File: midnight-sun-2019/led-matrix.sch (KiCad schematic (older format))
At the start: 826 parts

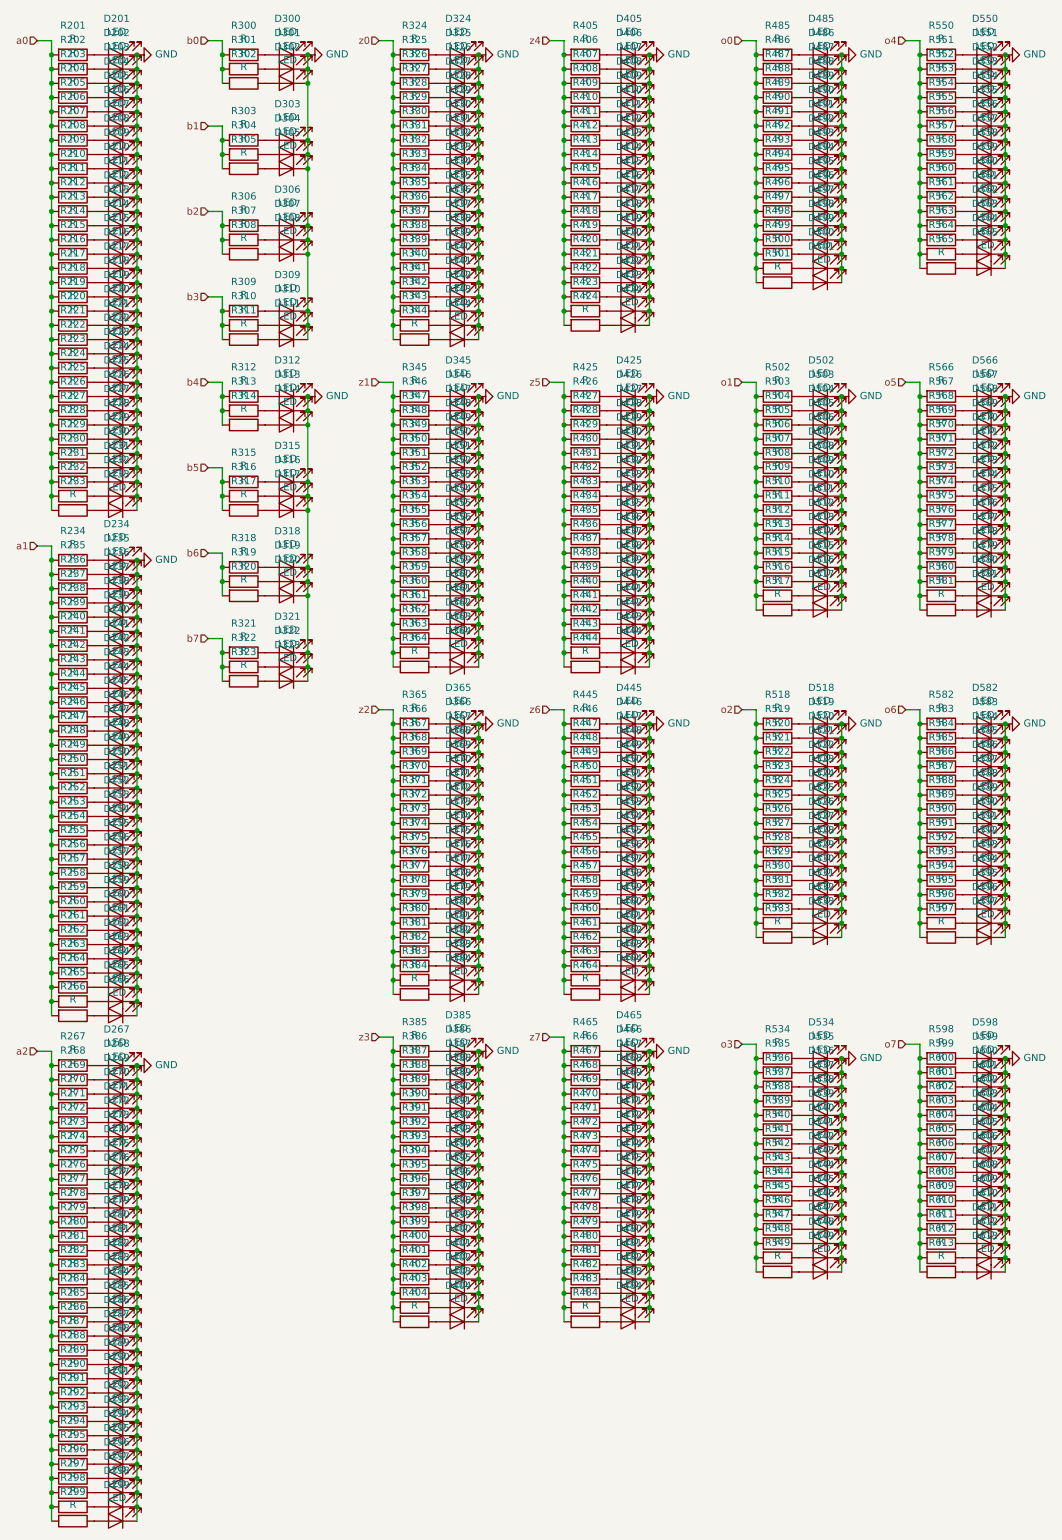
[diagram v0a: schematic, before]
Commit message: Clean up circuit draft
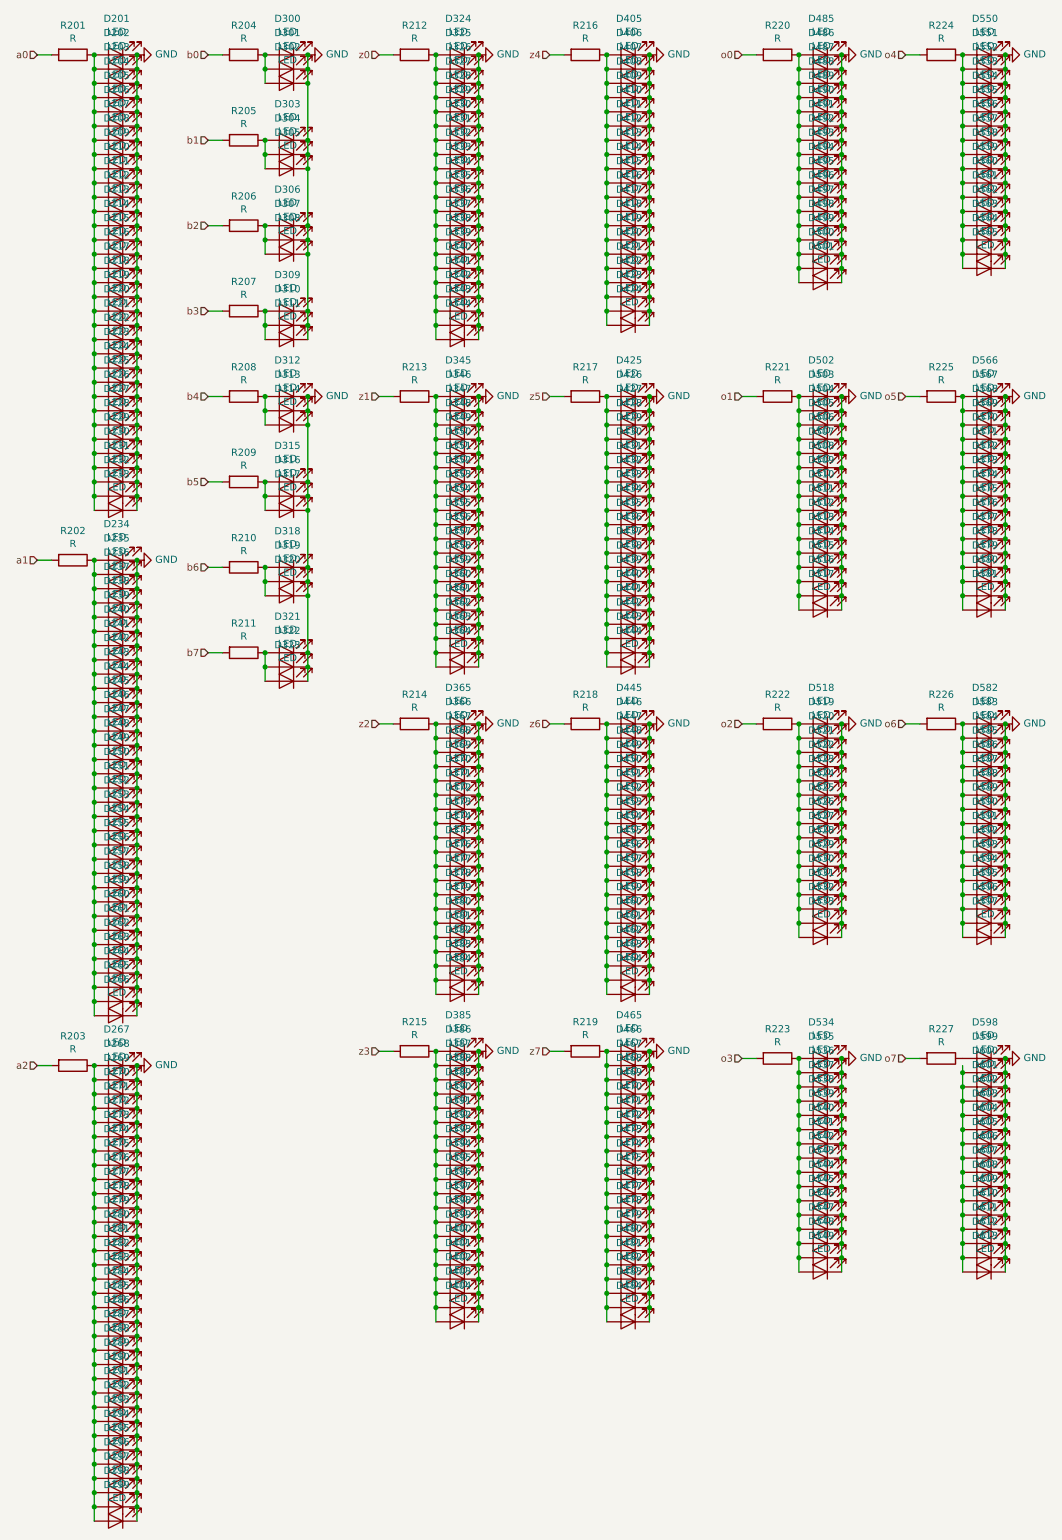
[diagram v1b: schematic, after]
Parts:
- removed R202, R203, R204, R205, R206, R207, R208, R209, R210, R211, R212, R213, R214, R215, R216, R217, R218, R219, R220, R221, R222, R223, R224, R225, R226, R227, R228, R229, R230, R231, R232, R233, R235, R236, R237, R238, R239, R240, R241, R242, R243, R244, R245, R246, R247, R248, R249, R250, R251, R252, R253, R254, R255, R256, R257, R258, R259, R260, R261, R262, R263, R264, R265, R266, R268, R269, R270, R271, R272, R273, R274, R275, R276, R277, R278, R279, R280, R281, R282, R283, R284, R285, R286, R287, R288, R289, R290, R291, R292, R293, R294, R295, R296, R297, R298, R299, R301, R302, R304, R305, R307, R308, R310, R311, R313, R314, R316, R317, R319, R320, R322, R323, R325, R326, R327, R328, R329, R330, R331, R332, R333, R334, R335, R336, R337, R338, R339, R340, R341, R342, R343, R344, R346, R347, R348, R349, R350, R351, R352, R353, R354, R355, R356, R357, R358, R359, R360, R361, R362, R363, R364, R366, R367, R368, R369, R370, R371, R372, R373, R374, R375, R376, R377, R378, R379, R380, R381, R382, R383, R384, R386, R387, R388, R389, R390, R391, R392, R393, R394, R395, R396, R397, R398, R399, R400, R401, R402, R403, R404, R406, R407, R408, R409, R410, R411, R412, R413, R414, R415, R416, R417, R418, R419, R420, R421, R422, R423, R424, R426, R427, R428, R429, R430, R431, R432, R433, R434, R435, R436, R437, R438, R439, R440, R441, R442, R443, R444, R446, R447, R448, R449, R450, R451, R452, R453, R454, R455, R456, R457, R458, R459, R460, R461, R462, R463, R464, R466, R467, R468, R469, R470, R471, R472, R473, R474, R475, R476, R477, R478, R479, R480, R481, R482, R483, R484, R486, R487, R488, R489, R490, R491, R492, R493, R494, R495, R496, R497, R498, R499, R500, R501, R503, R504, R505, R506, R507, R508, R509, R510, R511, R512, R513, R514, R515, R516, R517, R519, R520, R521, R522, R523, R524, R525, R526, R527, R528, R529, R530, R531, R532, R533, R535, R536, R537, R538, R539, R540, R541, R542, R543, R544, R545, R546, R547, R548, R549, R551, R552, R553, R554, R555, R556, R557, R558, R559, R560, R561, R562, R563, R564, R565, R567, R568, R569, R570, R571, R572, R573, R574, R575, R576, R577, R578, R579, R580, R581, R583, R584, R585, R586, R587, R588, R589, R590, R591, R592, R593, R594, R595, R596, R597, R599, R600, R601, R602, R603, R604, R605, R606, R607, R608, R609, R610, R611, R612, R613: R, symbol Device:R
- renumbered R234 to R202, R267 to R203, R300 to R204, R303 to R205, R306 to R206, R309 to R207, R312 to R208, R315 to R209, R318 to R210, R321 to R211, R324 to R212, R345 to R213, R365 to R214, R385 to R215, R405 to R216, R425 to R217, R445 to R218, R465 to R219, R485 to R220, R502 to R221, R518 to R222, R534 to R223, R550 to R224, R566 to R225, R582 to R226, R598 to R227
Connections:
- net at D612.2 (A): now also D599.2 (A), D600.2 (A), D601.2 (A), D602.2 (A), D603.2 (A), D604.2 (A), D605.2 (A), D606.2 (A), D607.2 (A), D608.2 (A), D609.2 (A), D610.2 (A), D611.2 (A), D613.2 (A)
- net at D596.2 (A): now also D582.2 (A), D583.2 (A), D584.2 (A), D585.2 (A), D586.2 (A), D587.2 (A), D588.2 (A), D589.2 (A), D590.2 (A), D591.2 (A), D592.2 (A), D593.2 (A), D594.2 (A), D595.2 (A), D597.2 (A), R226.1
- net at D580.2 (A): now also D566.2 (A), D567.2 (A), D568.2 (A), D569.2 (A), D570.2 (A), D571.2 (A), D572.2 (A), D573.2 (A), D574.2 (A), D575.2 (A), D576.2 (A), D577.2 (A), D578.2 (A), D579.2 (A), D581.2 (A), R225.1
- net at D564.2 (A): now also D550.2 (A), D551.2 (A), D552.2 (A), D553.2 (A), D554.2 (A), D555.2 (A), D556.2 (A), D557.2 (A), D558.2 (A), D559.2 (A), D560.2 (A), D561.2 (A), D562.2 (A), D563.2 (A), D565.2 (A), R224.1
- net at D548.2 (A): now also D534.2 (A), D535.2 (A), D536.2 (A), D537.2 (A), D538.2 (A), D539.2 (A), D540.2 (A), D541.2 (A), D542.2 (A), D543.2 (A), D544.2 (A), D545.2 (A), D546.2 (A), D547.2 (A), D549.2 (A), R223.1
- net at D532.2 (A): now also D518.2 (A), D519.2 (A), D520.2 (A), D521.2 (A), D522.2 (A), D523.2 (A), D524.2 (A), D525.2 (A), D526.2 (A), D527.2 (A), D528.2 (A), D529.2 (A), D530.2 (A), D531.2 (A), D533.2 (A), R222.1
- net at D516.2 (A): now also D502.2 (A), D503.2 (A), D504.2 (A), D505.2 (A), D506.2 (A), D507.2 (A), D508.2 (A), D509.2 (A), D510.2 (A), D511.2 (A), D512.2 (A), D513.2 (A), D514.2 (A), D515.2 (A), D517.2 (A), R221.1
- net at D501.2 (A): now also D485.2 (A), D486.2 (A), D487.2 (A), D488.2 (A), D489.2 (A), D490.2 (A), D491.2 (A), D492.2 (A), D493.2 (A), D494.2 (A), D495.2 (A), D496.2 (A), D497.2 (A), D498.2 (A), D499.2 (A), D500.2 (A), R220.1
- net at D484.2 (A): now also D465.2 (A), D466.2 (A), D467.2 (A), D468.2 (A), D469.2 (A), D470.2 (A), D471.2 (A), D472.2 (A), D473.2 (A), D474.2 (A), D475.2 (A), D476.2 (A), D477.2 (A), D478.2 (A), D479.2 (A), D480.2 (A), D481.2 (A), D482.2 (A), D483.2 (A), R219.1
- net at D464.2 (A): now also D445.2 (A), D446.2 (A), D447.2 (A), D448.2 (A), D449.2 (A), D450.2 (A), D451.2 (A), D452.2 (A), D453.2 (A), D454.2 (A), D455.2 (A), D456.2 (A), D457.2 (A), D458.2 (A), D459.2 (A), D460.2 (A), D461.2 (A), D462.2 (A), D463.2 (A), R218.1
- net at D444.2 (A): now also D425.2 (A), D426.2 (A), D427.2 (A), D428.2 (A), D429.2 (A), D430.2 (A), D431.2 (A), D432.2 (A), D433.2 (A), D434.2 (A), D435.2 (A), D436.2 (A), D437.2 (A), D438.2 (A), D439.2 (A), D440.2 (A), D441.2 (A), D442.2 (A), D443.2 (A), R217.1
- net at D424.2 (A): now also D405.2 (A), D406.2 (A), D407.2 (A), D408.2 (A), D409.2 (A), D410.2 (A), D411.2 (A), D412.2 (A), D413.2 (A), D414.2 (A), D415.2 (A), D416.2 (A), D417.2 (A), D418.2 (A), D419.2 (A), D420.2 (A), D421.2 (A), D422.2 (A), D423.2 (A), R216.1
- net at D404.2 (A): now also D385.2 (A), D386.2 (A), D387.2 (A), D388.2 (A), D389.2 (A), D390.2 (A), D391.2 (A), D392.2 (A), D393.2 (A), D394.2 (A), D395.2 (A), D396.2 (A), D397.2 (A), D398.2 (A), D399.2 (A), D400.2 (A), D401.2 (A), D402.2 (A), D403.2 (A), R215.1
- net at D384.2 (A): now also D365.2 (A), D366.2 (A), D367.2 (A), D368.2 (A), D369.2 (A), D370.2 (A), D371.2 (A), D372.2 (A), D373.2 (A), D374.2 (A), D375.2 (A), D376.2 (A), D377.2 (A), D378.2 (A), D379.2 (A), D380.2 (A), D381.2 (A), D382.2 (A), D383.2 (A), R214.1
- net at D364.2 (A): now also D345.2 (A), D346.2 (A), D347.2 (A), D348.2 (A), D349.2 (A), D350.2 (A), D351.2 (A), D352.2 (A), D353.2 (A), D354.2 (A), D355.2 (A), D356.2 (A), D357.2 (A), D358.2 (A), D359.2 (A), D360.2 (A), D361.2 (A), D362.2 (A), D363.2 (A), R213.1
- net at D344.2 (A): now also D324.2 (A), D325.2 (A), D326.2 (A), D327.2 (A), D328.2 (A), D329.2 (A), D330.2 (A), D331.2 (A), D332.2 (A), D333.2 (A), D334.2 (A), D335.2 (A), D336.2 (A), D337.2 (A), D338.2 (A), D339.2 (A), D340.2 (A), D341.2 (A), D342.2 (A), D343.2 (A), R212.1
- net at D312.2 (A), R208.1: now also D313.2 (A), D314.2 (A)
- net at D315.2 (A), R209.1: now also D316.2 (A), D317.2 (A)
- net at D318.2 (A), R210.1: now also D319.2 (A), D320.2 (A)
- net at D321.2 (A), R211.1: now also D322.2 (A), D323.2 (A)
- net at D300.2 (A), R204.1: now also D301.2 (A), D302.2 (A)
- net at D303.2 (A), R205.1: now also D304.2 (A), D305.2 (A)
- net at D306.2 (A), R206.1: now also D307.2 (A), D308.2 (A)
- net at D309.2 (A), R207.1: now also D310.2 (A), D311.2 (A)
- net at D299.2 (A): now also D267.2 (A), D268.2 (A), D269.2 (A), D270.2 (A), D271.2 (A), D272.2 (A), D273.2 (A), D274.2 (A), D275.2 (A), D276.2 (A), D277.2 (A), D278.2 (A), D279.2 (A), D280.2 (A), D281.2 (A), D282.2 (A), D283.2 (A), D284.2 (A), D285.2 (A), D286.2 (A), D287.2 (A), D288.2 (A), D289.2 (A), D290.2 (A), D291.2 (A), D292.2 (A), D293.2 (A), D294.2 (A), D295.2 (A), D296.2 (A), D297.2 (A), D298.2 (A), R203.1
- net at D266.2 (A): now also D234.2 (A), D235.2 (A), D236.2 (A), D237.2 (A), D238.2 (A), D239.2 (A), D240.2 (A), D241.2 (A), D242.2 (A), D243.2 (A), D244.2 (A), D245.2 (A), D246.2 (A), D247.2 (A), D248.2 (A), D249.2 (A), D250.2 (A), D251.2 (A), D252.2 (A), D253.2 (A), D254.2 (A), D255.2 (A), D256.2 (A), D257.2 (A), D258.2 (A), D259.2 (A), D260.2 (A), D261.2 (A), D262.2 (A), D263.2 (A), D264.2 (A), D265.2 (A), R202.1
- net at D233.2 (A): now also D201.2 (A), D202.2 (A), D203.2 (A), D204.2 (A), D205.2 (A), D206.2 (A), D207.2 (A), D208.2 (A), D209.2 (A), D210.2 (A), D211.2 (A), D212.2 (A), D213.2 (A), D214.2 (A), D215.2 (A), D216.2 (A), D217.2 (A), D218.2 (A), D219.2 (A), D220.2 (A), D221.2 (A), D222.2 (A), D223.2 (A), D224.2 (A), D225.2 (A), D226.2 (A), D227.2 (A), D228.2 (A), D229.2 (A), D230.2 (A), D231.2 (A), D232.2 (A), R201.1

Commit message: WIP: schematic
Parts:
- D201, D202, D203, D204, D205, D206, D207, D208, D209, D210, D211, D212, D213, D214, D215, D216, D217, D218, D219, D220, D221, D222, D223, D224, D225, D226, D227, D228, D229, D230, D231, D232, D233, D234, D235, D236, D237, D238, D239, D240, D241, D242, D243, D244, D245, D246, D247, D248, D249, D250, D251, D252, D253, D254, D255, D256, D257, D258, D259, D260, D261, D262, D263, D264, D265, D266, D267, D268, D269, D270, D271, D272, D273, D274, D275, D276, D277, D278, D279, D280, D281, D282, D283, D284, D285, D286, D287, D288, D289, D290, D291, D292, D293, D294, D295, D296, D297, D298, D299, D300, D301, D302, D303, D304, D305, D306, D307, D308, D309, D310, D311, D312, D313, D314, D315, D316, D317, D318, D319, D320, D321, D322, D323, D324, D325, D326, D327, D328, D329, D330, D331, D332, D333, D334, D335, D336, D337, D338, D339, D340, D341, D342, D343, D344, D345, D346, D347, D348, D349, D350, D351, D352, D353, D354, D355, D356, D357, D358, D359, D360, D361, D362, D363, D364, D365, D366, D367, D368, D369, D370, D371, D372, D373, D374, D375, D376, D377, D378, D379, D380, D381, D382, D383, D384, D385, D386, D387, D388, D389, D390, D391, D392, D393, D394, D395, D396, D397, D398, D399, D400, D401, D402, D403, D404, D405, D406, D407, D408, D409, D410, D411, D412, D413, D414, D415, D416, D417, D418, D419, D420, D421, D422, D423, D424, D425, D426, D427, D428, D429, D430, D431, D432, D433, D434, D435, D436, D437, D438, D439, D440, D441, D442, D443, D444, D445, D446, D447, D448, D449, D450, D451, D452, D453, D454, D455, D456, D457, D458, D459, D460, D461, D462, D463, D464, D465, D466, D467, D468, D469, D470, D471, D472, D473, D474, D475, D476, D477, D478, D479, D480, D481, D482, D483, D484, D485, D486, D487, D488, D489, D490, D491, D492, D493, D494, D495, D496, D497, D498, D499, D500, D501, D502, D503, D504, D505, D506, D507, D508, D509, D510, D511, D512, D513, D514, D515, D516, D517, D518, D519, D520, D521, D522, D523, D524, D525, D526, D527, D528, D529, D530, D531, D532, D533, D534, D535, D536, D537, D538, D539, D540, D541, D542, D543, D544, D545, D546, D547, D548, D549, D550, D551, D552, D553, D554, D555, D556, D557, D558, D559, D560, D561, D562, D563, D564, D565, D566, D567, D568, D569, D570, D571, D572, D573, D574, D575, D576, D577, D578, D579, D580, D581, D582, D583, D584, D585, D586, D587, D588, D589, D590, D591, D592, D593, D594, D595, D596, D597, D598, D599, D600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: footprint (none) -> LED_SMD:LED_0805_2012Metric_Castellated
- R201, R202, R203, R204, R205, R206, R207, R208, R209, R210, R211, R212, R213, R214, R215, R216, R217, R218, R219, R220, R221, R222, R223, R224, R225, R226, R227: footprint (none) -> Resistor_SMD:R_0805_2012Metric_Pad1.15x1.40mm_HandSolder
